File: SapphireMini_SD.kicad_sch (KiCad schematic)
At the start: 15 parts, among them J301 503182-1852, U301 MB85RS1MT, U302 TPS22860DBVR

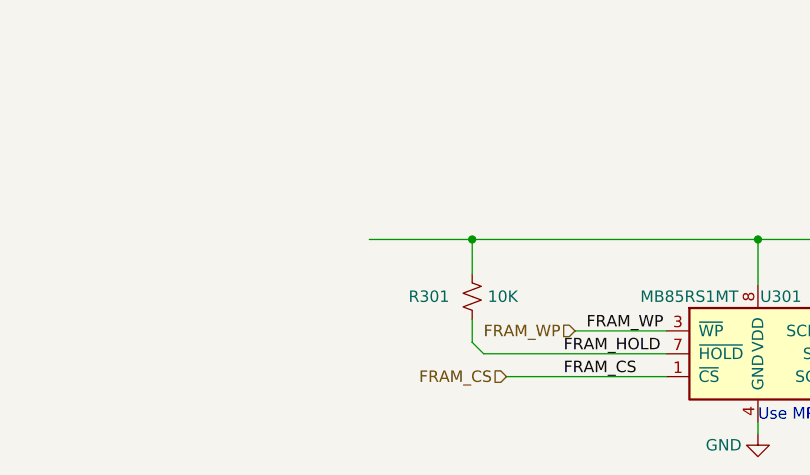
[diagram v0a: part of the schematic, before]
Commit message: Working on update to power controllers
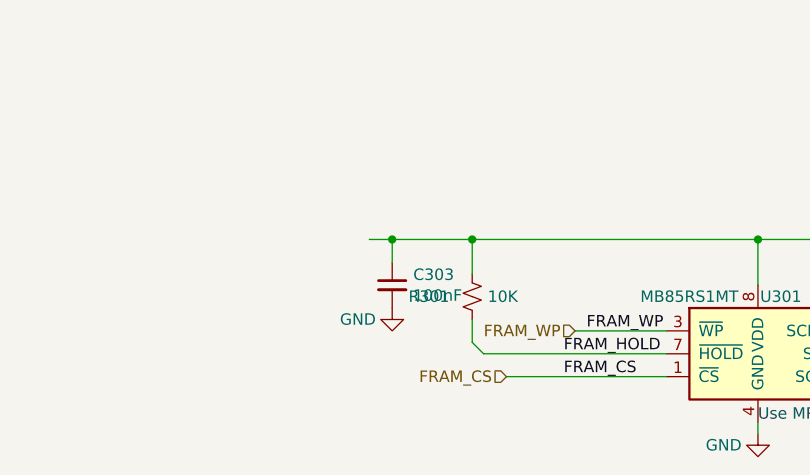
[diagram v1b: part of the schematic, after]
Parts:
- added C303: 100nF, Capacitor_SMD:C_0603_1608Metric, symbol Device:C_Small
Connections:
- net GND: now also C303.2
- net P3V3: now also C303.1
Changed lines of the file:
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@@
   (junction (at 102.87 135.89) (diameter 0) (color 0 0 0 0)
   )
+  (junction (at 62.23 135.89) (diameter 0) (color 0 0 0 0)
+  )
   (junction (at 92.71 81.28) (diameter 0) (color 0 0 0 0)
   )
@@
     (stroke (width 0) (type default) (color 0 0 0 0))
   )
-  (wire (pts (xy 71.12 135.89) (xy 59.69 135.89))
+  (wire (pts (xy 71.12 135.89) (xy 62.23 135.89))
     (stroke (width 0) (type default) (color 0 0 0 0))
   )
@@
     (stroke (width 0) (type default) (color 0 0 0 0))
   )
+  (wire (pts (xy 62.23 135.89) (xy 59.69 135.89))
+    (stroke (width 0) (type default) (color 0 0 0 0))
+  )
   (wire (pts (xy 220.98 62.23) (xy 219.71 60.96))
     (stroke (width 0) (type default) (color 0 0 0 0))
@@
   )
   (wire (pts (xy 199.39 97.79) (xy 199.39 95.25))
+    (stroke (width 0) (type default) (color 0 0 0 0))
+  )
+  (wire (pts (xy 62.23 138.43) (xy 62.23 135.89))
     (stroke (width 0) (type default) (color 0 0 0 0))
   )
@@
     (pin "6")
   )
+  (symbol (lib_id "power:GND") (at 62.23 143.51 0) (mirror y) (unit 1)
+    (in_bom yes) (on_board yes)
+    (property "Reference" "#PWR0307" (id 0) (at 62.23 149.86 0)
+      (effects (font (size 1.27 1.27)) hide)
+    )
+    (property "Value" "GND" (id 1) (at 58.42 144.78 0))
+    (property "Footprint" "" (id 2) (at 62.23 143.51 0)
+      (effects (font (size 1.27 1.27)) hide)
+    )
+    (property "Datasheet" "" (id 3) (at 62.23 143.51 0)
+      (effects (font (size 1.27 1.27)) hide)
+    )
+    (pin "1")
+  )
   (symbol (lib_id "Device:R_US") (at 207.01 73.66 270) (unit 1)
     (in_bom yes) (on_board yes)
@@
       (effects (font (size 1.27 1.27)) hide)
     )
+    (pin "1")
+    (pin "2")
+  )
+  (symbol (lib_id "Device:C_Small") (at 62.23 140.97 0) (unit 1)
+    (in_bom yes) (on_board yes)
+    (property "Reference" "C303" (id 0) (at 64.5668 139.8016 0)
+      (effects (font (size 1.27 1.27)) (justify left))
+    )
+    (property "Value" "100nF" (id 1) (at 64.5668 142.113 0)
+      (effects (font (size 1.27 1.27)) (justify left))
+    )
+    (property "Footprint" "Capacitor_SMD:C_0603_1608Metric" (id 2) (at 62.23 140.97 0)
+      (effects (font (size 1.27 1.27)) hide)
+    )
+    (property "Datasheet" "~" (id 3) (at 62.23 140.97 0)
+      (effects (font (size 1.27 1.27)) hide)
+    )
+    (property "DigiKey Price" "0.10" (id 4) (at 62.23 140.97 0)
+      (effects (font (size 1.27 1.27)) hide)
+    )
+    (property "MPN" "CL05A104KA5NNNC" (id 5) (at 62.23 140.97 0)
+      (effects (font (size 1.27 1.27)) hide)
+    )
+    (property "Manufacturer" "Samsung" (id 6) (at 62.23 140.97 0)
+      (effects (font (size 1.27 1.27)) hide)
+    )
+    (property "Tolerance" "10%" (id 7) (at 62.23 140.97 0)
+      (effects (font (size 1.27 1.27)) hide)
+    )
+    (property "Voltage" "25" (id 8) (at 62.23 140.97 0)
+      (effects (font (size 1.27 1.27)) hide)
+    )
+    (property "Voltage Rating (DC)" "25 volt" (id 9) (at 62.23 140.97 0)
+      (effects (font (size 1.27 1.27)) hide)
+    )
+    (property "Populate" "1" (id 10) (at 62.23 140.97 0)
+      (effects (font (size 1.27 1.27)) hide)
+    )
+    (property "MacroFab_PN" "MF-CAP-0603-0.1uF" (id 11) (at 62.23 140.97 0)
+      (effects (font (size 1.27 1.27)) hide)
+    )
+    (property "Digi-Key_PN" "1276-1006-1-ND " (id 12) (at 62.23 140.97 0)
+      (effects (font (size 1.27 1.27)) hide)
+    )
+    (property "Distributor" "Digikey" (id 13) (at 62.23 140.97 0)
+      (effects (font (size 1.27 1.27)) hide)
+    )
+    (property "DPN" "1276-1006-1-ND " (id 14) (at 62.23 140.97 0)
+      (effects (font (size 1.27 1.27)) hide)
+    )
+    (property "Description" "0.1 µF ±10% 25V Ceramic Capacitor X5R 0402 (1005 Metric)" (id 15) (at 62.23 140.97 0)
+      (effects (font (size 1.27 1.27)) hide)
+    )

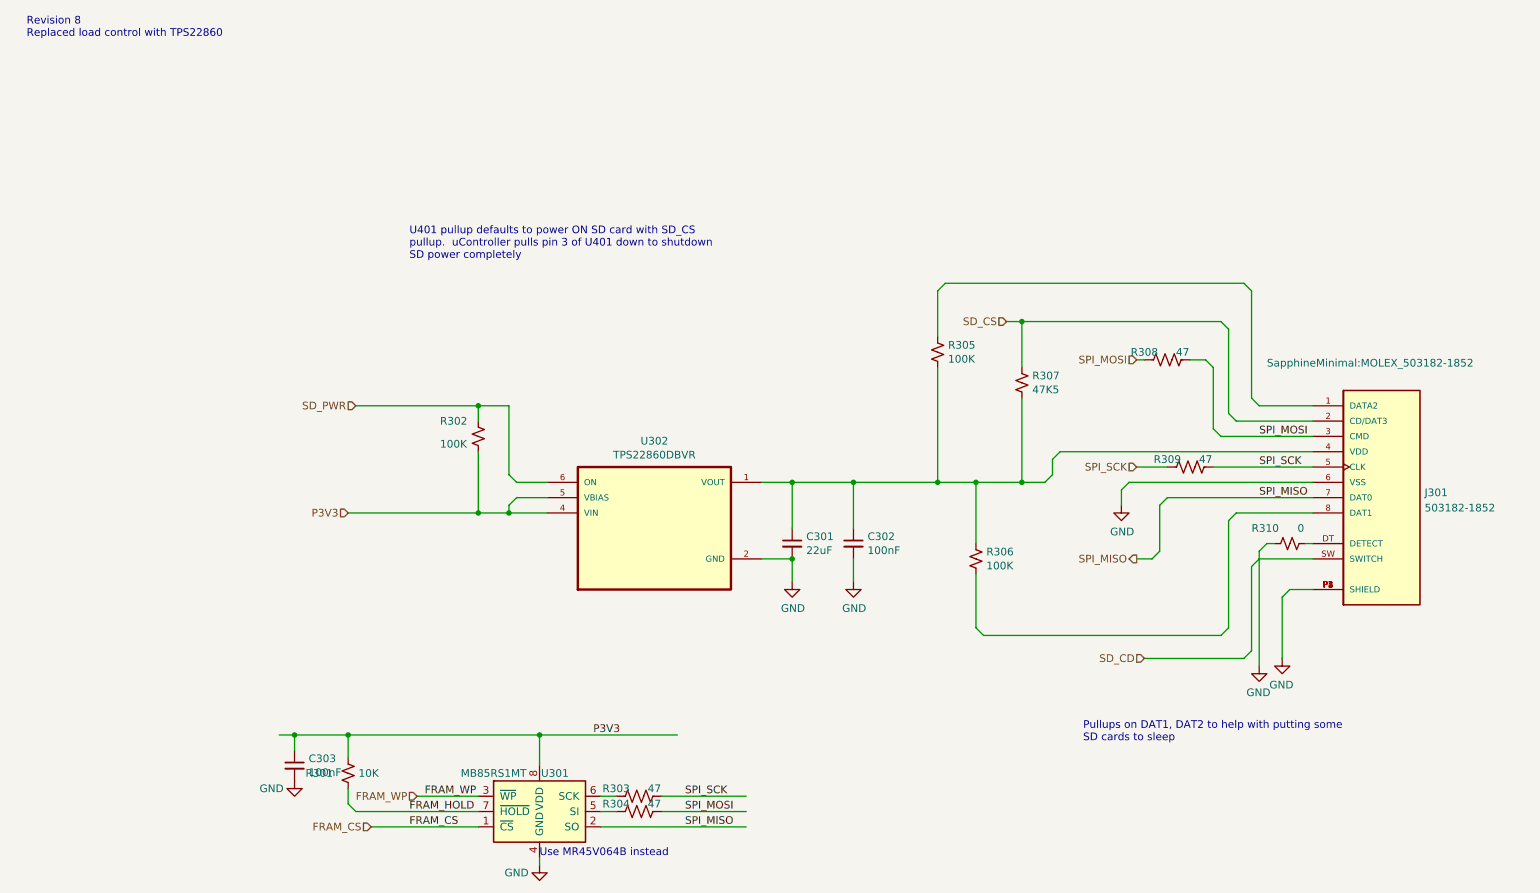
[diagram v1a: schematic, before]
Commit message: Checkpoint
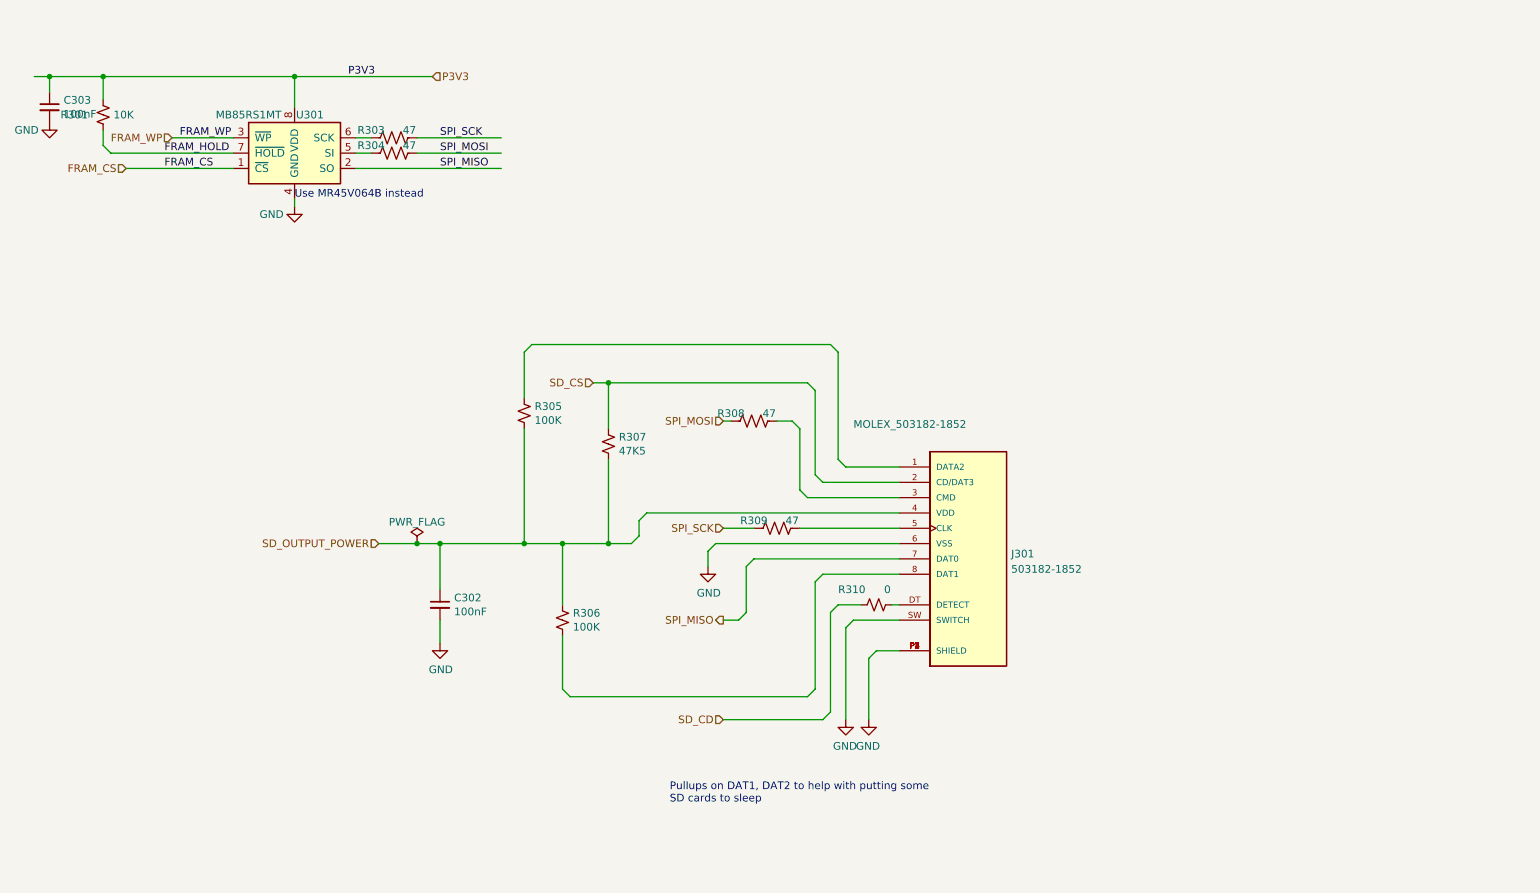
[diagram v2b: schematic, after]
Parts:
- removed C301: 22uF, Capacitor_SMD:C_1206_3216Metric, symbol Device:C_Small
- removed R302: 100K, Resistor_SMD:R_0603_1608Metric, symbol Device:R_Small_US
- removed U302: TPS22860DBVR, SOT95P280X145-6N, symbol sapphireMini:TPS22860DBVR
- J301: footprint SapphineMinimal:MOLEX_503182-1852 -> MOLEX_503182-1852
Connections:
- net GND: now also J301.SW (SWITCH); no longer R310.1
- net SD_CD: now also R310.1; no longer J301.SW (SWITCH)
- net SPI_MOSI: no longer J301.3 (CMD), R308.1
- net SPI_SCK: no longer J301.5 (CLK), R309.1
- net SD_OUTPUT_POWER: now reaches C302.1, J301.4 (VDD), R305.2, R306.1, R307.1
- new net: J301.3 (CMD), R308.1
- new net: J301.5 (CLK), R309.1
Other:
- note removed: "Revision 8 Replaced load control with TPS22860"
- note removed: "U401 pullup defaults to power ON SD card with SD_CS pullup. uController pulls pin 3 of U401 down to shutdown SD power completely"
- moved on the sheet: C302, C303, J301, R301, R303, R304, R305, R306, R307, R308, R309, R310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
